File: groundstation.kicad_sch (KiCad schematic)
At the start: 10 parts, among them J1 USB_C_Receptacle_USB2.0_16P, J2 62684-402100ALF, SW1 SW_Push, U1 ESP32-S3-WROOM-1

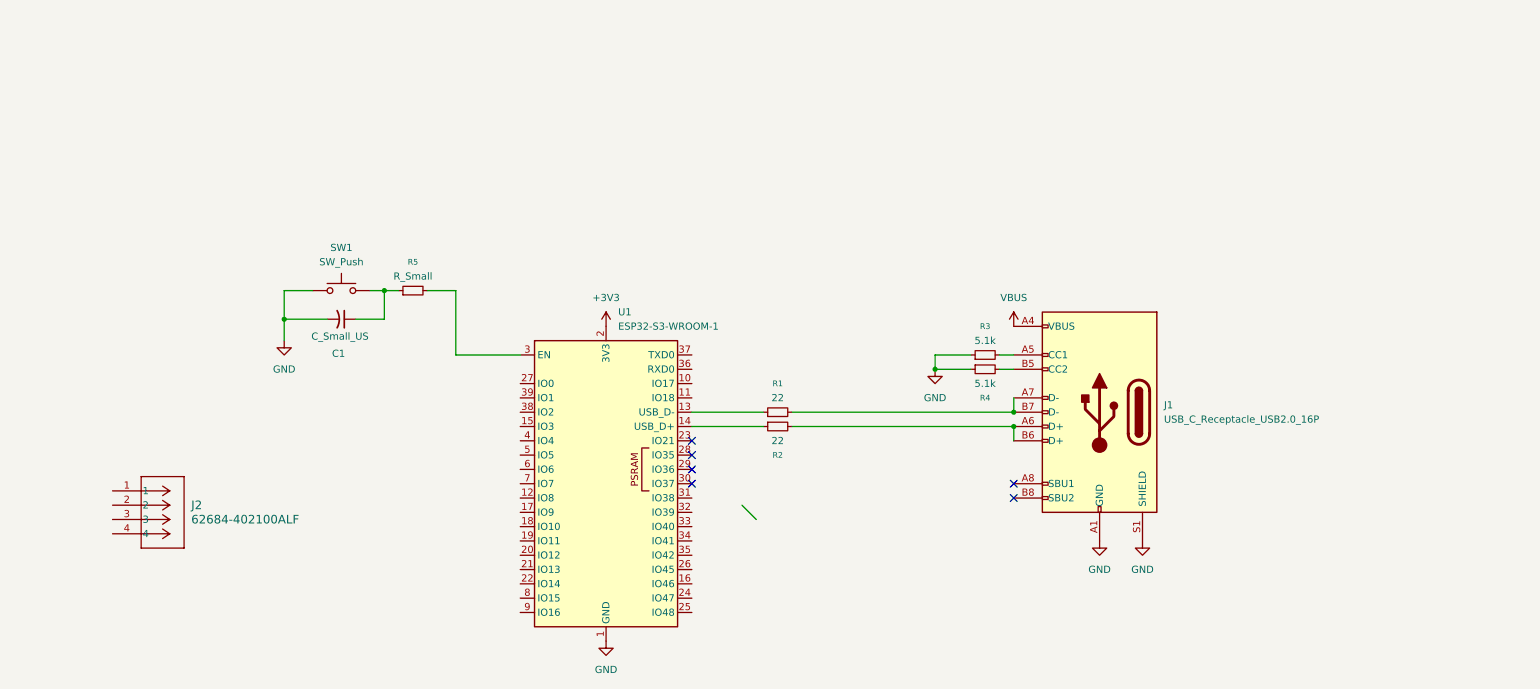
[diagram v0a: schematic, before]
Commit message: Update schematicand PCB
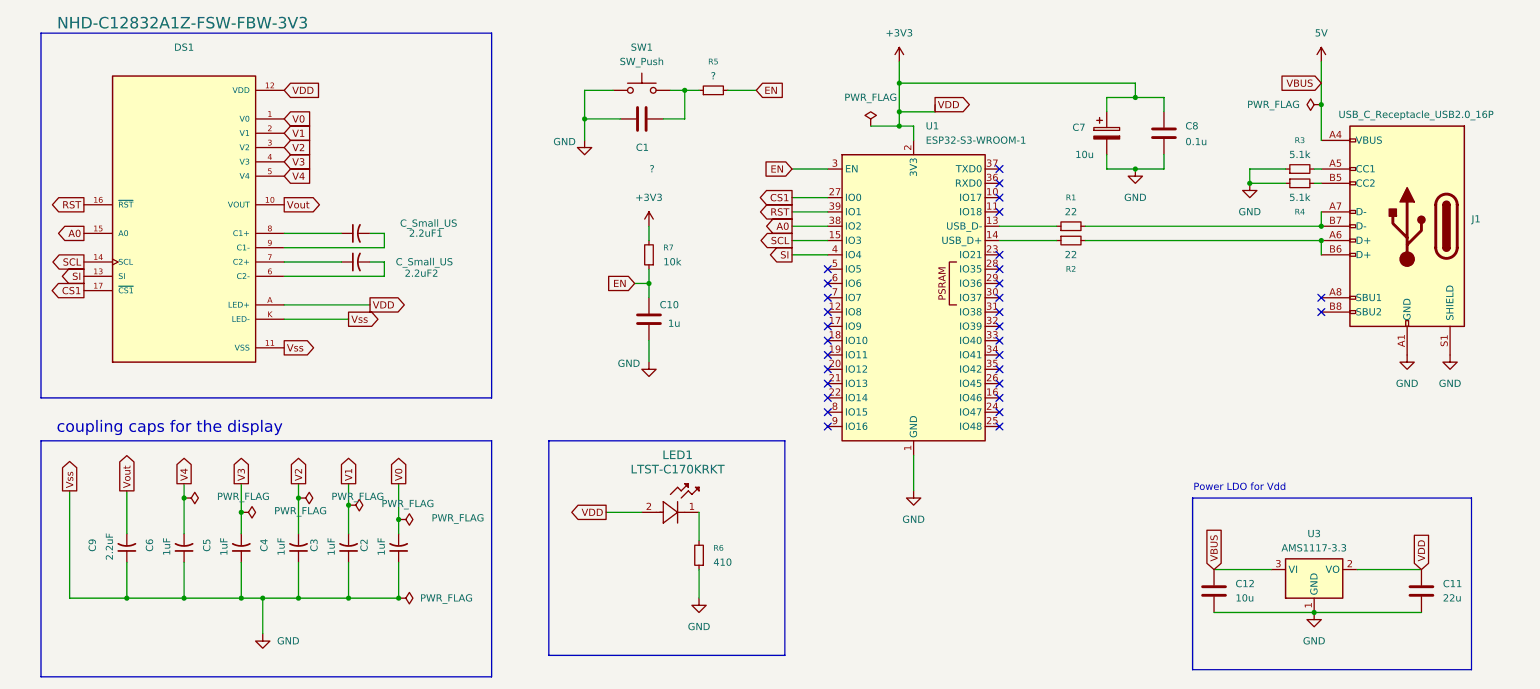
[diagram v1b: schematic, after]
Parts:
- removed C1: C_Small_US, Capacitor_THT:C_Disc_D3.0mm_W1.6mm_P2.50mm, symbol Device:C_Small_US
- removed J2: 62684-402100ALF, CONN_62684-402100ALF_AMP, symbol FCC 40 0.5mm:62684-402100ALF
- added 2.2uF1, 2.2uF2: C_Small_US, Capacitor_SMD:C_0402_1005Metric, symbol Device:C_Small_US
- added C1: ?, symbol Device:C
- added C10: 1u, symbol Device:C
- added C11: 22u, Capacitor_SMD:C_0603_1608Metric, symbol Device:C
- added C12: 10u, symbol Device:C
- added C2, C3, C4, C5, C6: 1uF, Capacitor_SMD:C_0402_1005Metric, symbol Device:C_Small_US
- added C7: 10u, symbol Device:C_Polarized
- added C8: 0.1u, symbol Device:C
- added C9: 2.2uF, Capacitor_SMD:C_0402_1005Metric, symbol Device:C_Small_US
- added DS1: NHD-C12832A1Z-FSW-FBW-3V3, Ground_Station:LCD_NHD-C12832A1Z-FSW-FBW-3V3, symbol NHD LCD display:NHD-C12832A1Z-FSW-FBW-3V3
- added LED1: LTST-C170KRKT, Ground_Station:LED_LTST-C170KRKT_LTO-M, symbol LTST-C170krkt:LTST-C170KRKT
- added R6: 410, symbol Device:R_Small
- added R7: 10k, Resistor_SMD:R_0402_1005Metric, symbol Device:R_Small
- added U3: AMS1117-3.3, Package_TO_SOT_SMD:SOT-223-3_TabPin2, symbol Regulator_Linear:AMS1117-3.3
- R5: value R_Small -> ?; footprint Capacitor_THT:C_Disc_D3.0mm_W1.6mm_P2.50mm -> Resistor_SMD:R_0402_1005Metric
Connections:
- net +3V3: now also C11.1, C7.1, C8.1, DS1.12 (VDD), DS1.A (LED+), LED1.2, R7.2, U3.2 (VO)
- net GND: now also C1.1, C10.1, C11.2, C12.2, C2.1, C3.1, C4.1, C5.1, C6.1, C7.2, C8.2, C9.1, DS1.11 (VSS), DS1.K (LED-), R6.1, U3.1 (GND)
- net at R5.1, SW1.2: now also C1.2
- net SCL: now reaches U1.15 (IO3)
- net SCL: now also DS1.14 (SCL)
- net CS1: now reaches U1.27 (IO0)
- net CS1: now also DS1.17 (~{CS1})
- net EN: now reaches R5.2, U1.3 (EN)
- net EN: now also C10.2, R7.1
- net A0: now reaches U1.38 (IO2)
- net A0: now also DS1.15 (A0)
- net RST: now reaches U1.39 (IO1)
- net RST: now also DS1.16 (~{RST})
- net SI: now reaches U1.4 (IO4)
- net SI: now also DS1.13 (SI)
- net VBUS renamed 5V
- net 5V: now also C12.1, U3.3 (VI)
- new net: LED1.1, R6.2
- new net: 2.2uF2.2, DS1.6 (C2-)
- new net: 2.2uF2.1, DS1.7 (C2+)
- new net: 2.2uF1.1, DS1.8 (C1+)
- new net: 2.2uF1.2, DS1.9 (C1-)
- new net V0: C2.2, DS1.1 (V0)
- new net V1: C3.2, DS1.2 (V1)
- new net V2: C4.2, DS1.3 (V2)
- new net V3: C5.2, DS1.4 (V3)
- new net V4: C6.2, DS1.5 (V4)
- new net Vout: C9.2, DS1.10 (VOUT)
- no-connect marks 6 -> 31
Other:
- note added: "Power LDO for Vdd"
- note added: "coupling caps for the display"
- moved on the sheet: J1, R1, R2, R3, R4, R5, SW1, U1
